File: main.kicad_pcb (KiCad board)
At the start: 2 copper layers, 31.3 x 52.8 mm, 21 parts

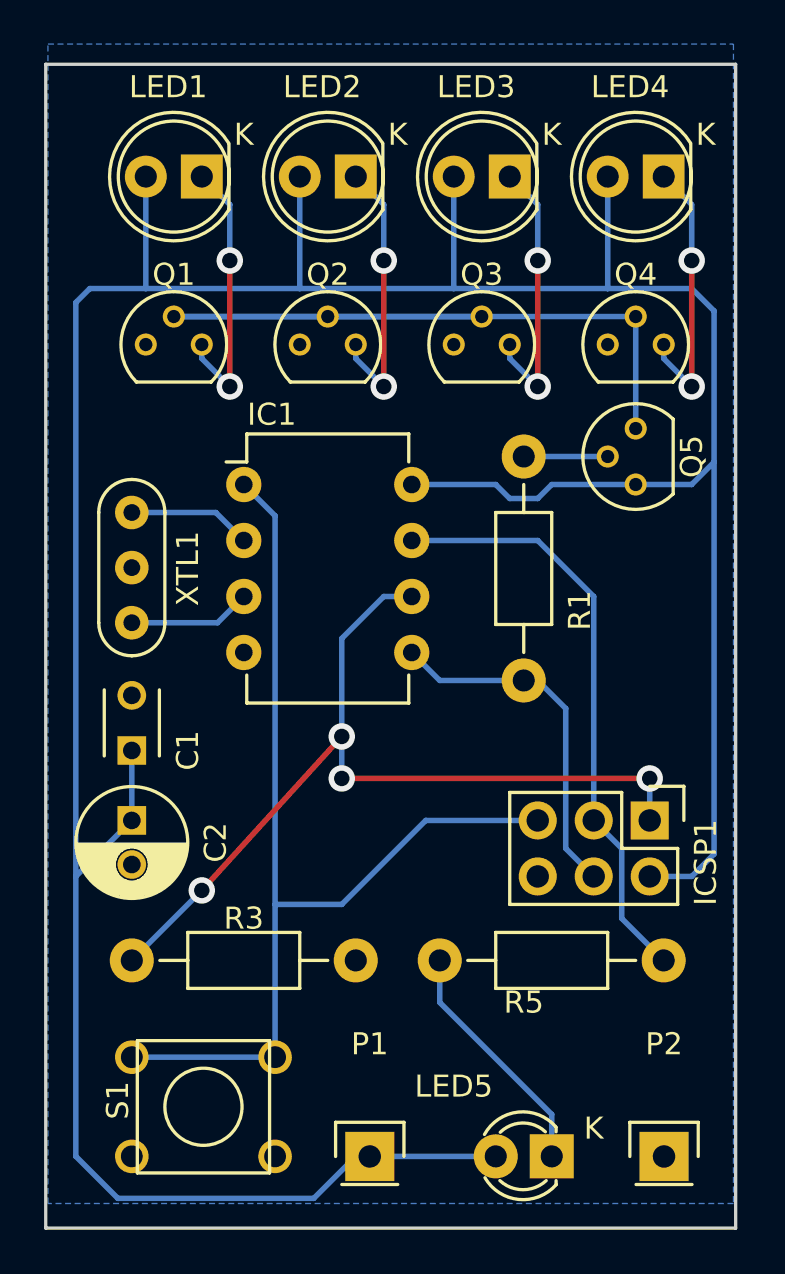
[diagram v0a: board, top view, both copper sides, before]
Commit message: last so far
yes pls
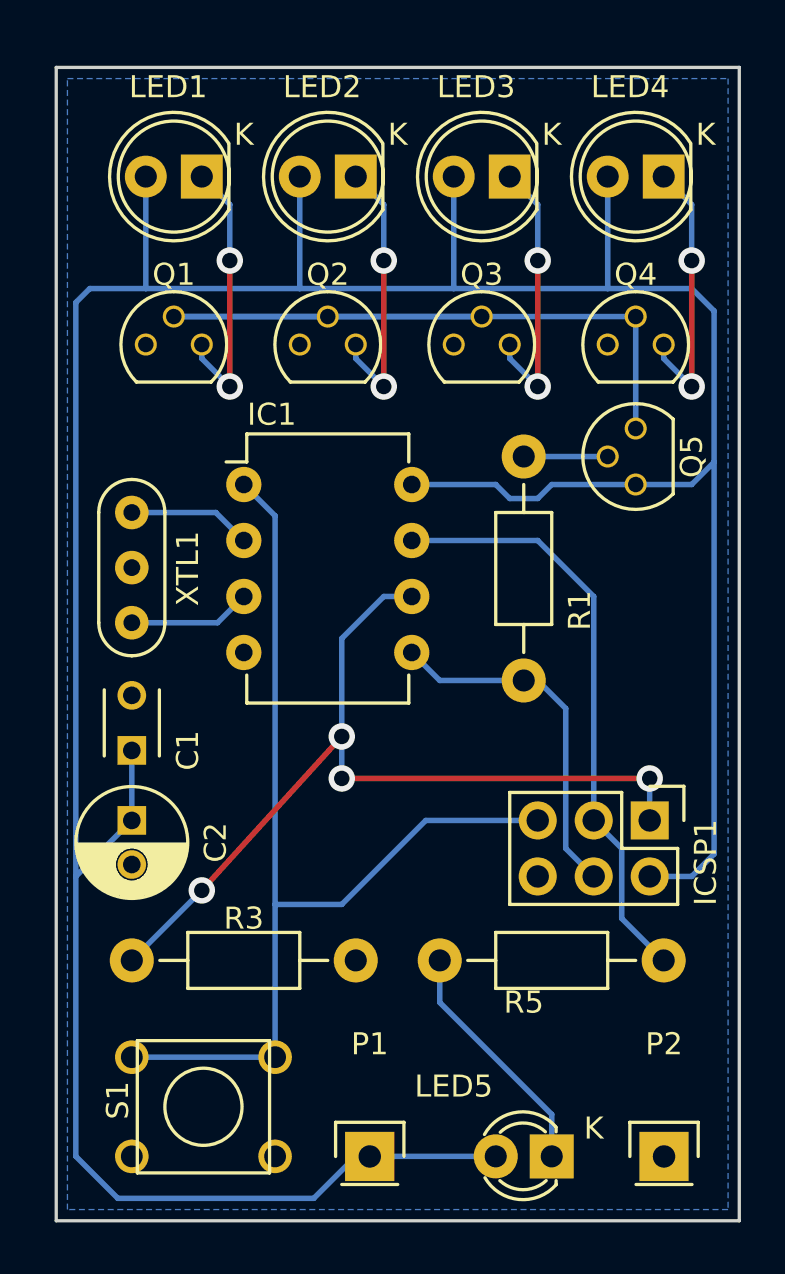
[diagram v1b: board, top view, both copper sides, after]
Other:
- board size 31.3 x 52.8 mm -> 31 x 52.3 mm
- net class Default: trace_width 0.25 -> 0.5
